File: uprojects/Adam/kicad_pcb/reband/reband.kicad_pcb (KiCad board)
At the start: 2 copper layers, 3 parts, among them U1 ESP32-C3FH4, U2 LMV324MT, U3 MAX30009ENA+T

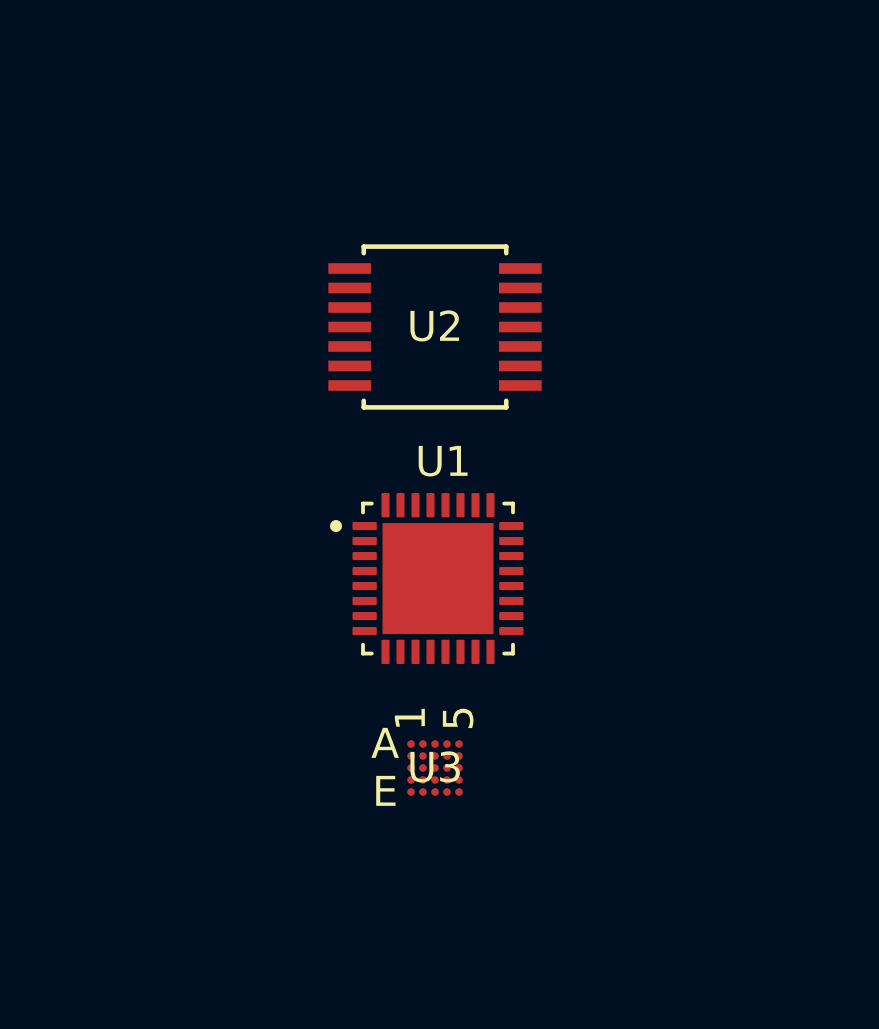
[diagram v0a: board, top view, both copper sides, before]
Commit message: ROOM 25 MAY 2026 Updates
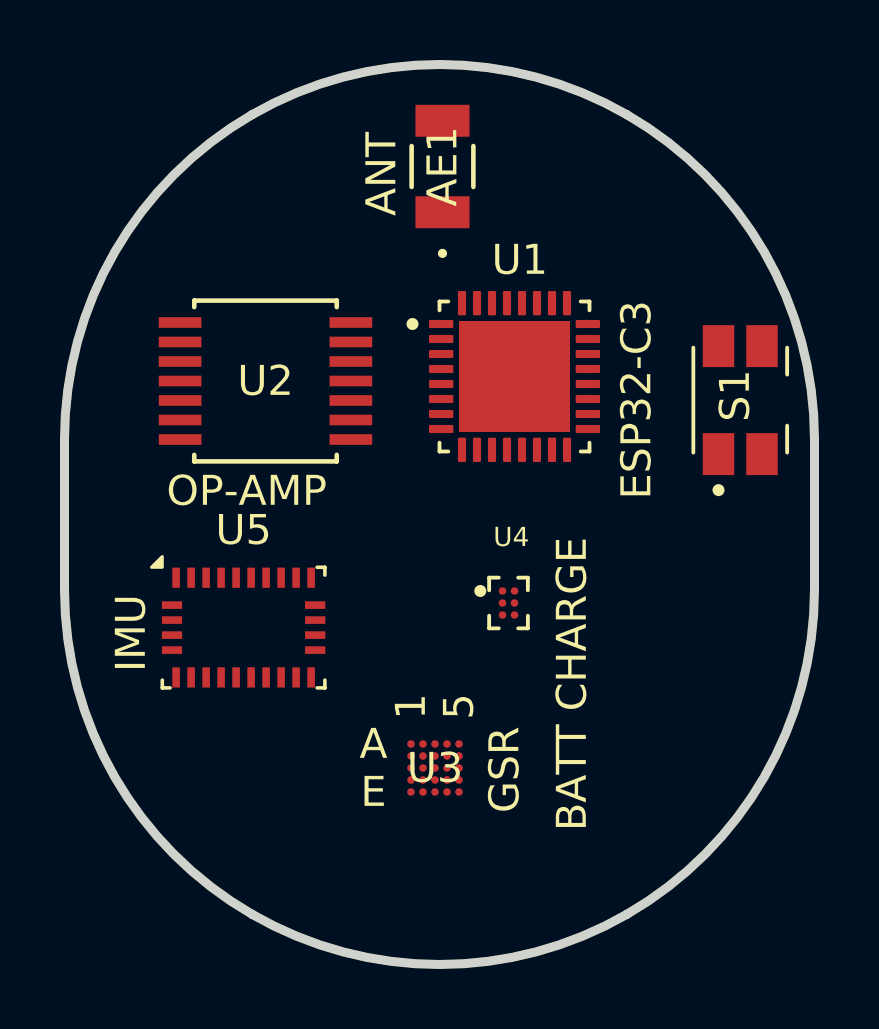
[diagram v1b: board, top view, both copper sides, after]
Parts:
- added AE1: AMCA31-2R450G-S1F-T3, AMCA31_2R450G_S1F_T3:ANT_AMCA31-2R450G-S1F-T3_ABR, F.Cu at (139.8, 77.7)
- added S1: EVQ-P7A01P, EVQ_P7A01P:SW_EVQ-P7A01P, F.Cu at (149.7, 85.4)
- added U4: BQ25100YFPR, BQ25100YFPR:BGA6N40P3X2_157X88X50N, F.Cu at (141.9, 92.2)
- added U5: BNO055, Package_LGA:LGA-28_5.2x3.8mm_P0.5mm, F.Cu at (133.1, 93.0)
- moved U1 7.20 mm to (142.2, 84.7)
- moved U2 5.93 mm to (133.8, 84.8)
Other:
- board outline added: 25 x 30 mm
- board text added: "ANT"
- board text added: "BATT CHARGE"
- board text added: "ESP32-C3"
- board text added: "GSR"
- board text added: "IMU"
- board text added: "OP-AMP"
